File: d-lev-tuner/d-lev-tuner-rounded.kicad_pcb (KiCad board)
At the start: 4 copper layers, 88.7 x 68.4 mm, 39 parts, among them J1 S6B-PH-SM4-TB, U1 STP08CP05, U2 STP08CP05, U3 AP2112K-3.3, U4 STP08CP05, U5 DSM7TA56

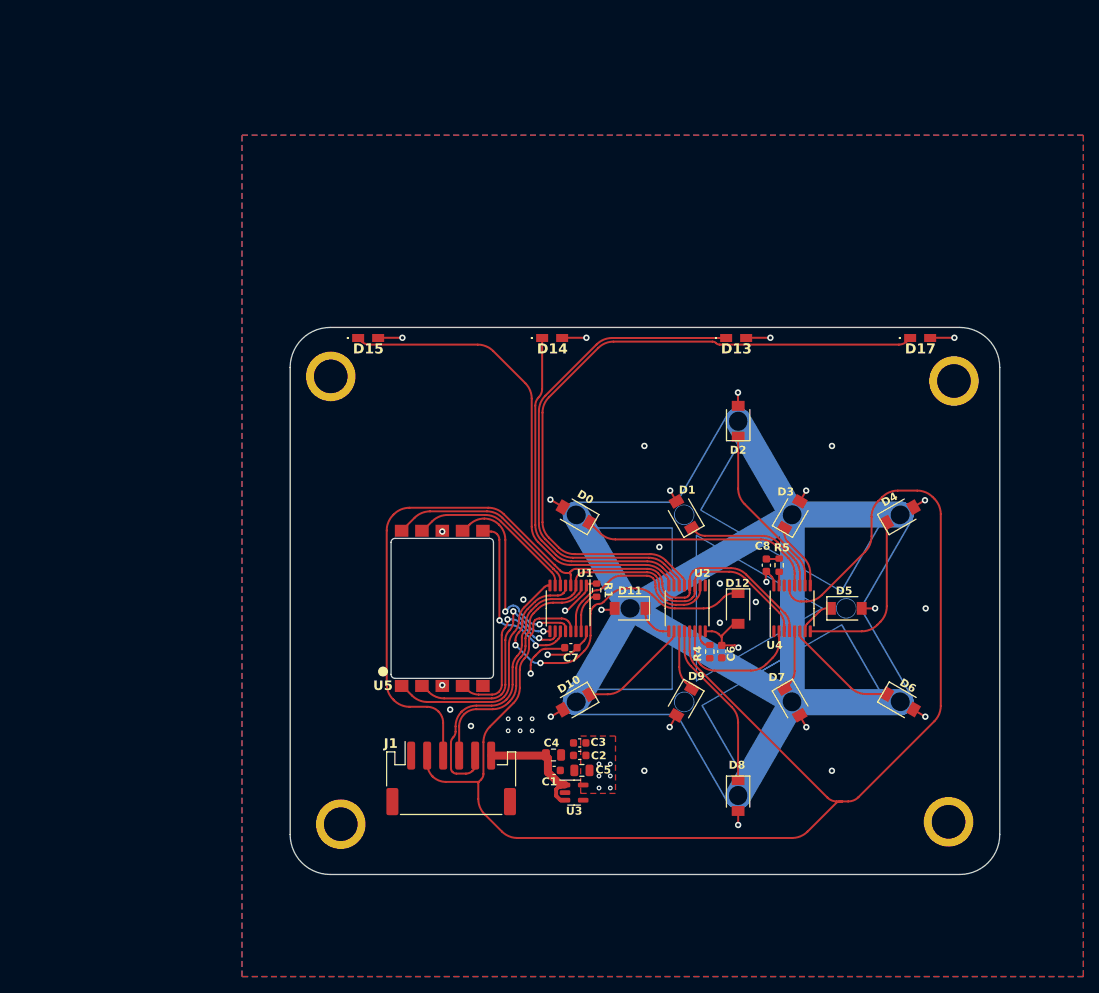
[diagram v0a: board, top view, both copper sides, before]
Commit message: all design files updated with current contents of jlc cart
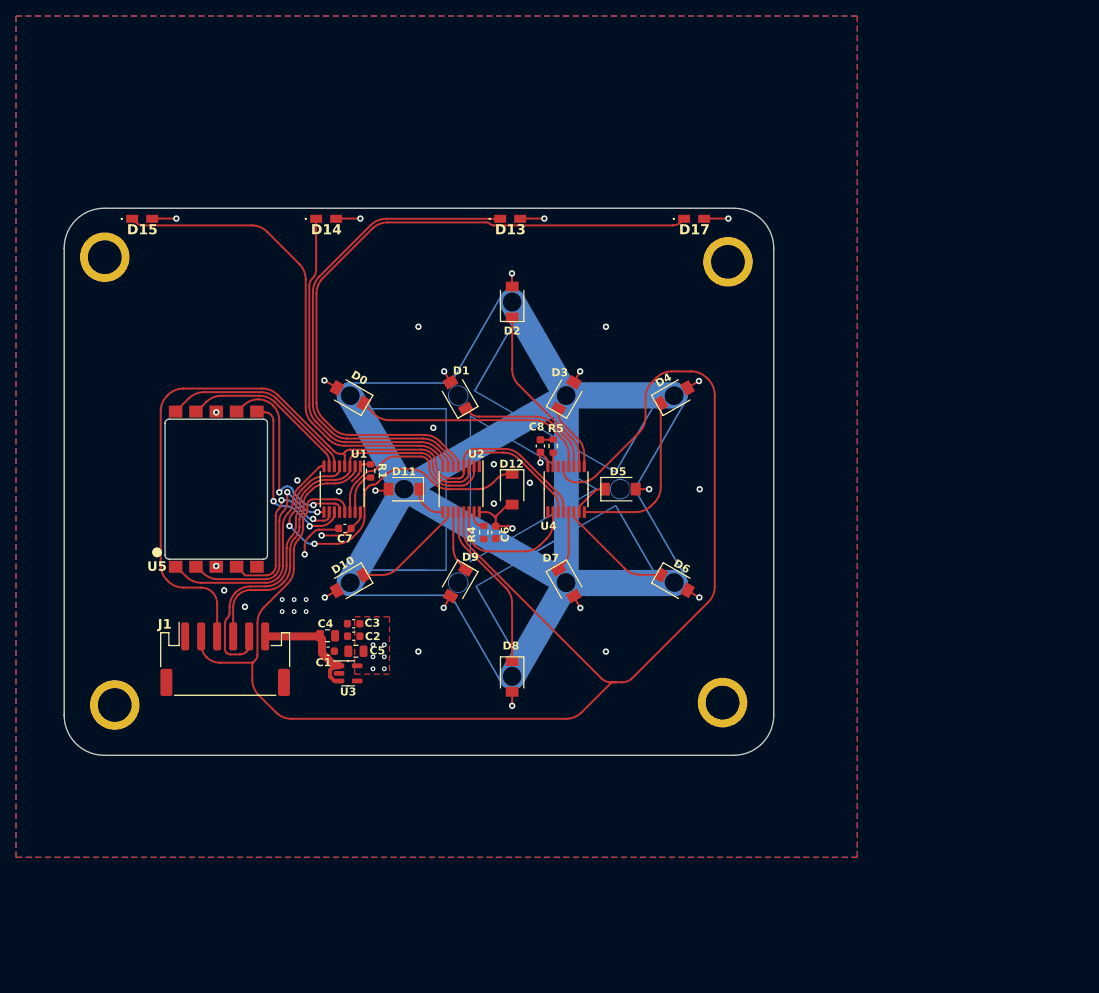
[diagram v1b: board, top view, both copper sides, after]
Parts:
- added G***: LOGO, LOGO, F.Cu at (35.4, 30.3)
- moved D14 31.9 mm to (48.6, 17.7)
- moved J1 31.9 mm to (36.0, 72.8)
- moved U1 31.9 mm to (50.6, 51.5)
- moved C1 31.9 mm to (48.9, 71.8)
- moved C6 31.9 mm to (69.8, 56.9)
- moved C8 31.9 mm to (75.4, 46.1)
- moved D0 31.9 mm to (51.7, 39.8)
- moved D1 31.9 mm to (65.2, 39.8)
- moved D10 31.9 mm to (51.7, 63.2)
- moved D12 31.9 mm to (71.9, 51.5)
- moved D13 31.9 mm to (71.7, 17.7)
- moved D15 31.9 mm to (25.6, 17.7)
- moved D17 31.9 mm to (94.7, 17.7)
- moved D2 31.9 mm to (71.9, 28.1)
- moved D3 31.9 mm to (78.6, 39.8)
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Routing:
- net GND: track 13.5 -> 11.8 mm
- net C: track 22.0 -> 22.9 mm
